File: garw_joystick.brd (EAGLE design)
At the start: 45 x 30 mm, 15 parts, among them IC1 TLC339D, X1 PS-05_WL, X2 PS-08_WL

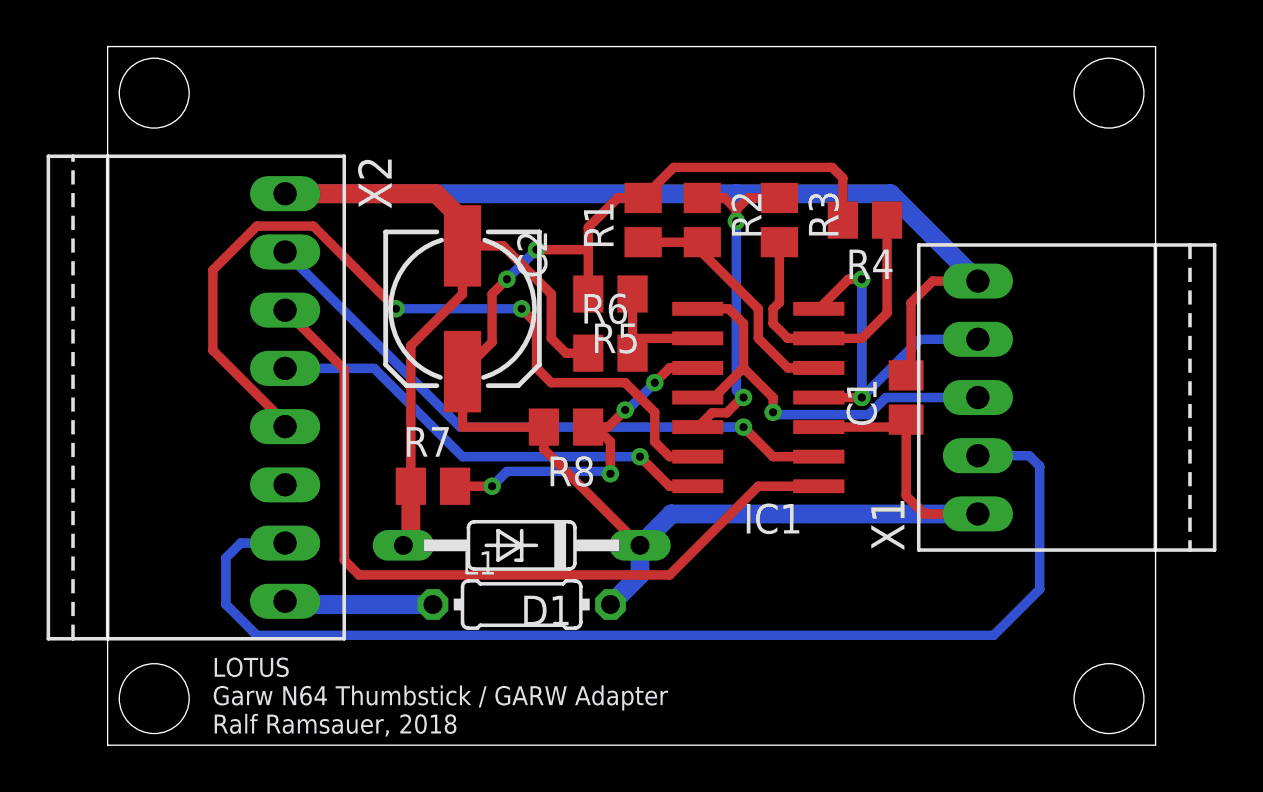
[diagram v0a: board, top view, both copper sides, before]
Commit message: Improve board
Signed-off-by: Ralf Ramsauer <ralf@vmexit.de>
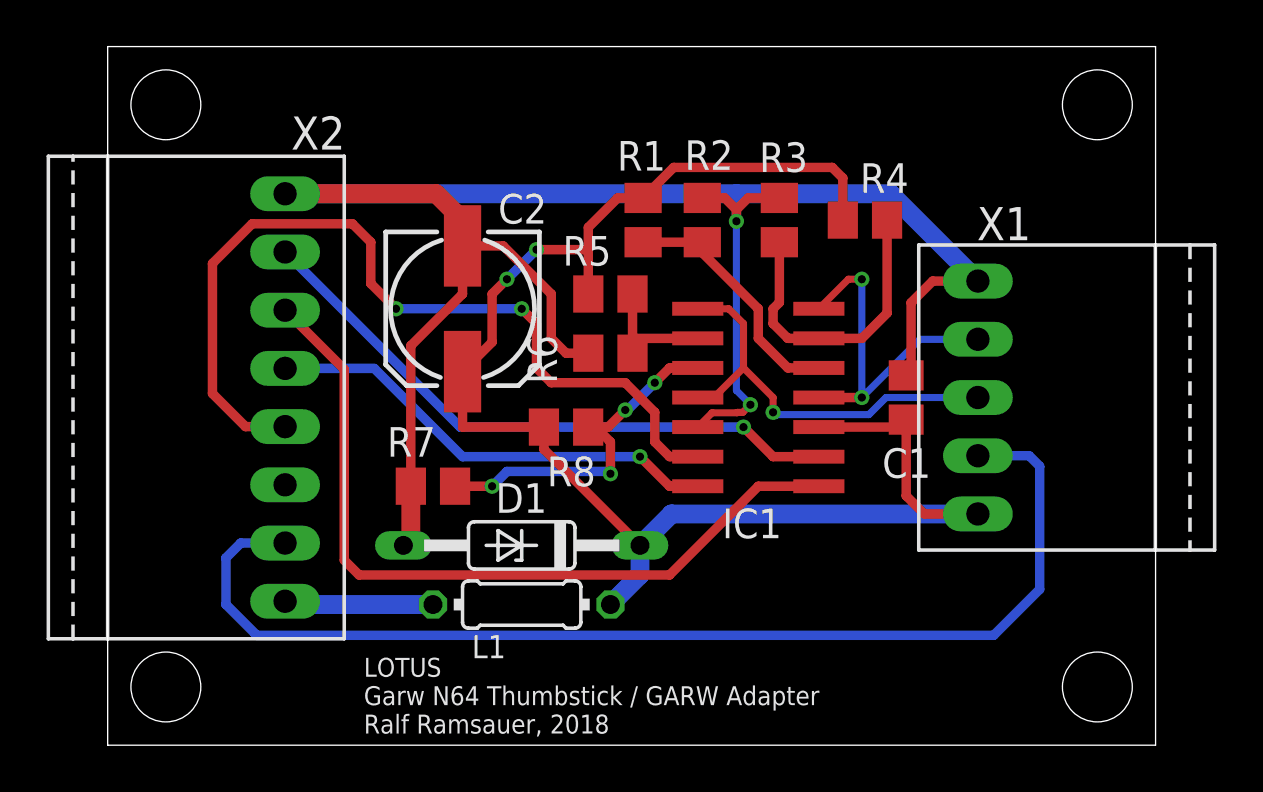
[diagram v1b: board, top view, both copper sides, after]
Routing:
- net GARW4: track 35.6 -> 37.9 mm
- net GND: track 84.9 -> 85.5 mm
